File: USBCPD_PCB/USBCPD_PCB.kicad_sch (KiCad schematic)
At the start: 64 parts, among them IC1 TMCS1108A3BQDRQ1, IC2 UCC27282QDRQ1, IC3 UCC27282QDRQ1, IC4 BAJ2CC0FP-E2, J1 TB002-500-02BE, J2 TB002-500-02BE, Q1 SIR584DP-T1-RE3, Q2 SIR584DP-T1-RE3, Q3 SIR584DP-T1-RE3, Q4 SIR584DP-T1-RE3, U1 NUCLEO-G474RE

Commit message: schematic rewire changes & hotfixes
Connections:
- net PB12_LED: no longer U1.CN10_16 (PB12)
- net PB13_PWM: now also R2.1; no longer R7.1
- net PC2_ADC_Vout: now reaches U1.CN7_35 (PC2)
- net PC2_ADC_Vout: now also R13.2, R14.1
- net PC3_ADC_Iout: now reaches U1.CN7_37 (PC3)
- net PC3_ADC_Iout: now also R5.2
- net PB15_PWM: now reaches U1.CN10_26 (PB15)
- net PB15_PWM: now also R7.1
- removed net PA10_ADC_Vout: R13.2, R14.1, U1.CN10_33 (PA10)
- net PA8_PWM renamed PA8_LED
- net PA8_LED: no longer R2.1
- net PA9_PWM: no longer names the net of U1.CN10_21 (PA9)
- net PA9_PWM: no longer R1.1
- net PB3_ADC_Iout: no longer names the net of U1.CN10_31 (PB3)
- net PB3_ADC_Iout: no longer R5.2
- new net PB12_PWM: R1.1, U1.CN10_16 (PB12)

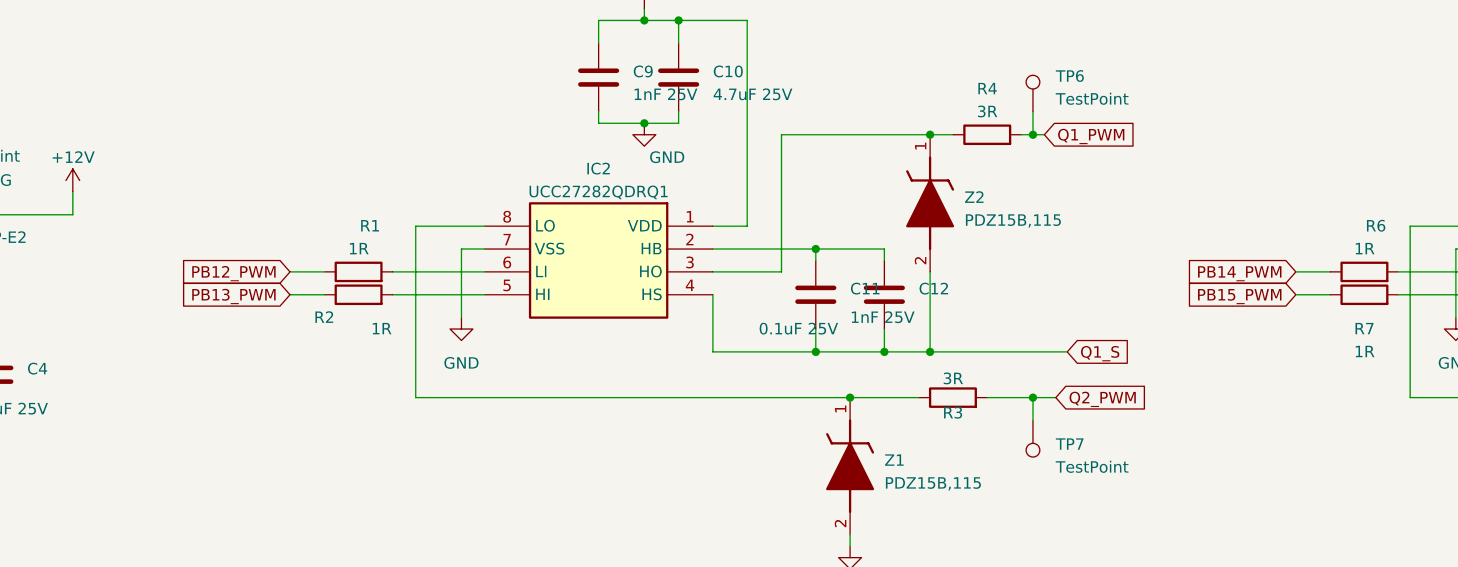
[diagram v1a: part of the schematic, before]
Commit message: save
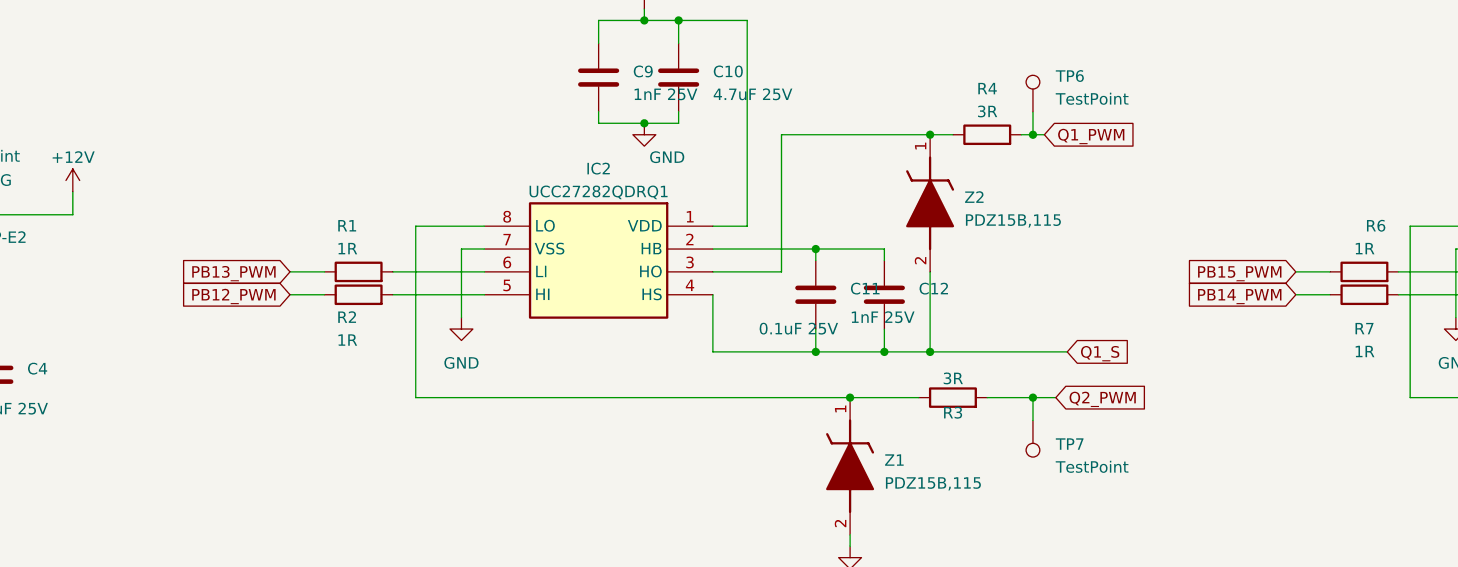
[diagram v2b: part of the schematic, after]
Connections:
- net PB12_PWM: now also R2.1; no longer R1.1
- net PB13_PWM: now also R1.1; no longer R2.1
- net PB14_PWM: now also R7.1; no longer R6.1
- net PB15_PWM: now also R6.1; no longer R7.1
